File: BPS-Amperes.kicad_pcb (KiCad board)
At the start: 2 copper layers, 40 x 50 mm, 35 parts, among them J1 Conn_02x10_Odd_Even, J2 ShuntConn, J3 PassthroughConn, J4 TestConn, J5 Conn_01x02, U1 INA186A3IDDFT, U2 OPA2196, U4 REF1930AIDDCT

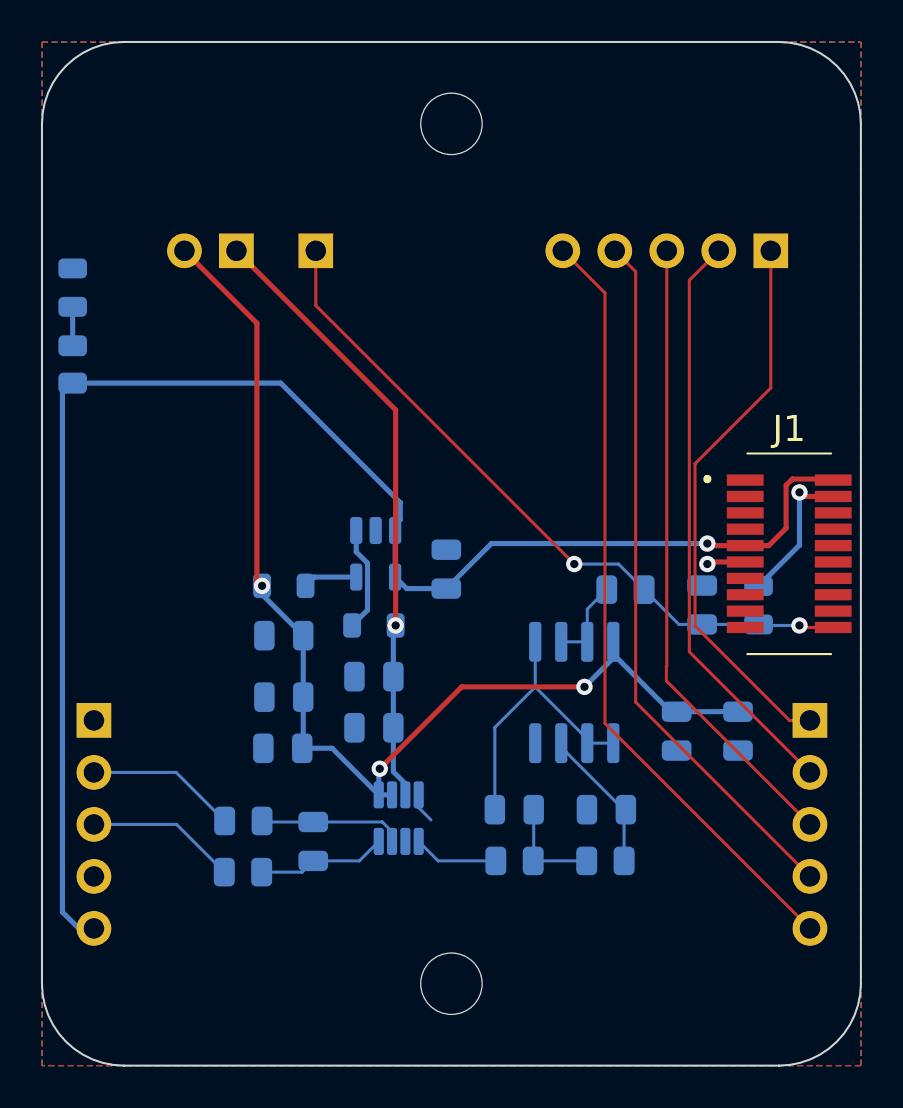
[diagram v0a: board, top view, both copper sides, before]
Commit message: The Thickening
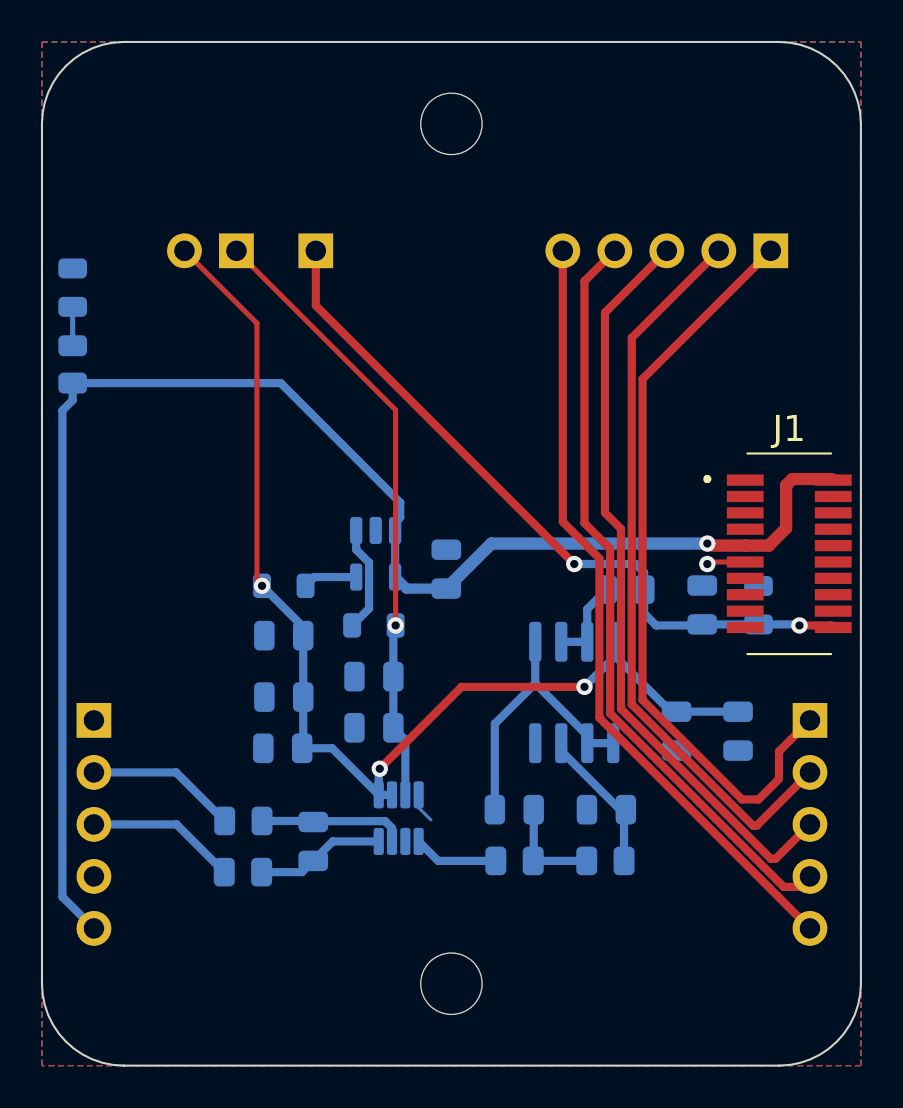
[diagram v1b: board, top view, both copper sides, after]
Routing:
- net /NOTCON: track 27.4 -> 37.1 mm
- net /SHUNT: track 28.5 -> 36.2 mm
- net GND: track 18.2 -> 11.1 mm, vias 2 -> 1
- net /TEST: track 30.9 -> 36.9 mm
- net /V+: track 34.5 -> 37.2 mm
- net /PA1: track 34.5 -> 35.7 mm
- net +3V0: track 55.7 -> 55.0 mm
